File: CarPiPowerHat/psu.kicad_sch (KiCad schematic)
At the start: 42 parts, among them J5 USB_A, Q1 DMMT5401, Q2 DMG2305UX, Q3 DMP3013SFV-7, U1 AP64501SP-13, U6 RT9742SNGV

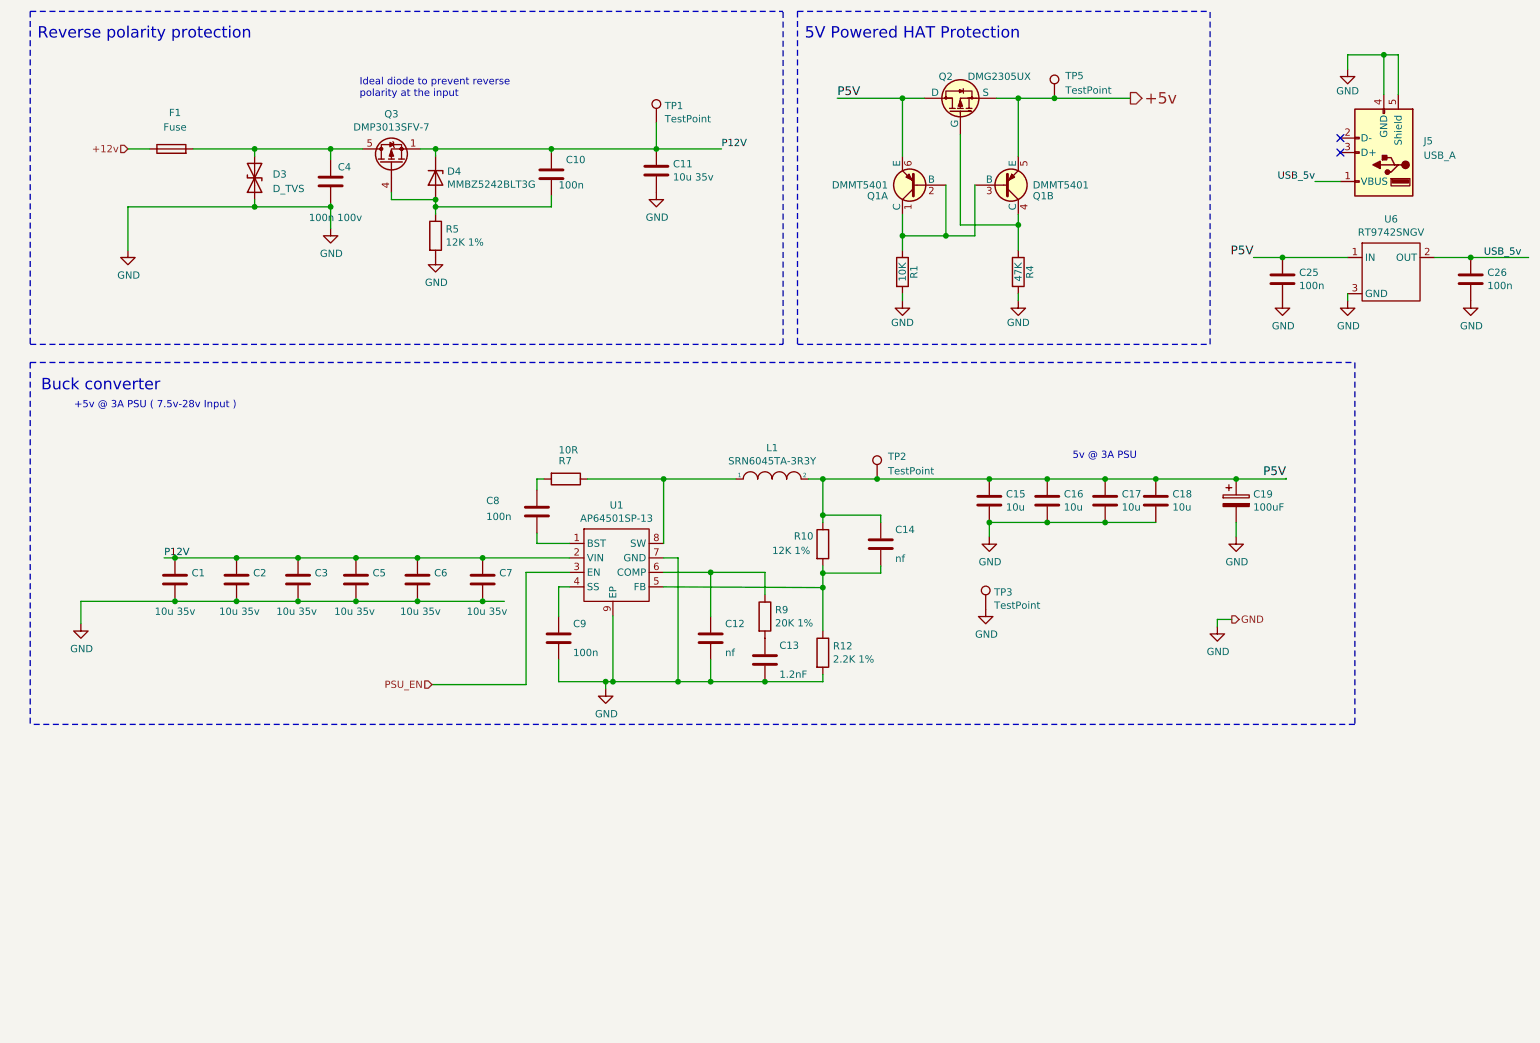
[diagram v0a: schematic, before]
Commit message: Everything routed, DRC ok
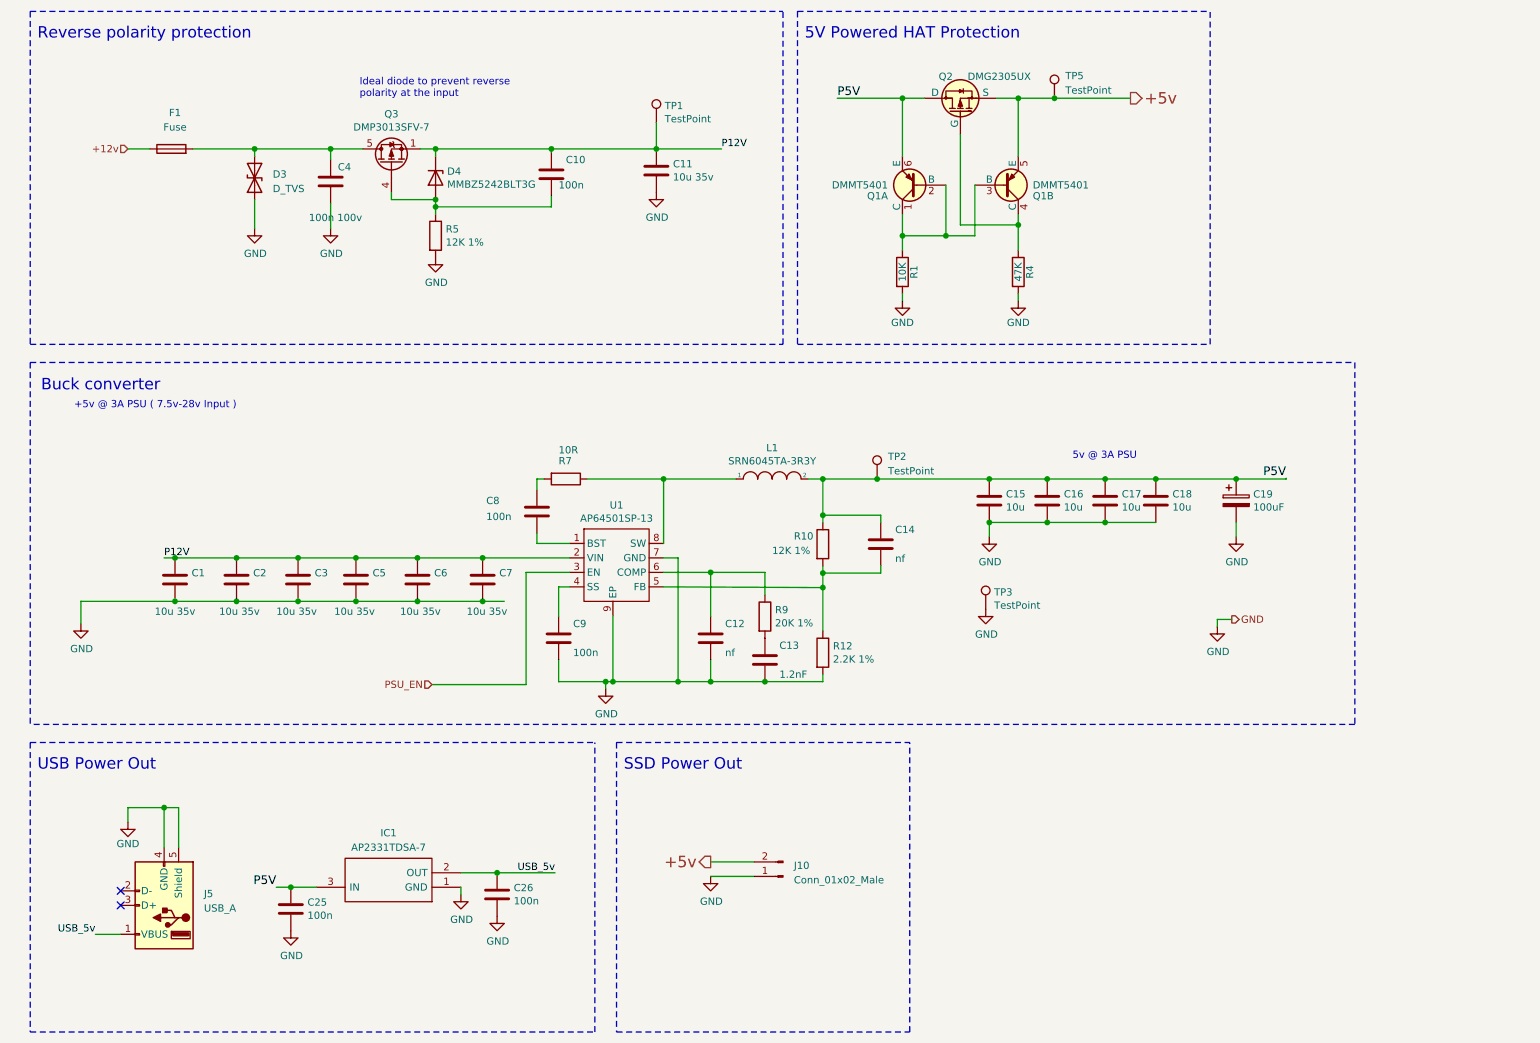
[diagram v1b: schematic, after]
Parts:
- removed U6: RT9742SNGV, Package_TO_SOT_SMD:SOT-23, symbol CM4IO:RT9742SNGV
- added IC1: AP2331TDSA-7, ap2331:SOT96P240X110-3N, symbol AP2331TDSA-7:AP2331TDSA-7
- added J10: Conn_01x02_Male, Connector_JST:JST_XH_S2B-XH-A_1x02_P2.50mm_Horizontal, symbol Connector:Conn_01x02_Male
- C10, C25, C26, C4: LCSC (none) -> C1525
- C11: LCSC (none) -> C469541
- D4: LCSC (none) -> C268585
- Q1: LCSC (none) -> C154733
- Q2: LCSC (none) -> C144153
- R5: LCSC (none) -> C25879
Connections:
- net +5v: now also J10.2 (Pin_2)
- net GND: now also IC1.1 (GND), J10.1 (Pin_1)
- net P5V: now also IC1.3 (IN)
- net USB_5v: now also IC1.2 (OUT)
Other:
- note added: "SSD Power Out"
- note added: "USB Power Out"
- moved on the sheet: C25, C26, J5
